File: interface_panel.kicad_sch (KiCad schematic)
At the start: 5 parts, among them J1 Conn_02x04_Odd_Even

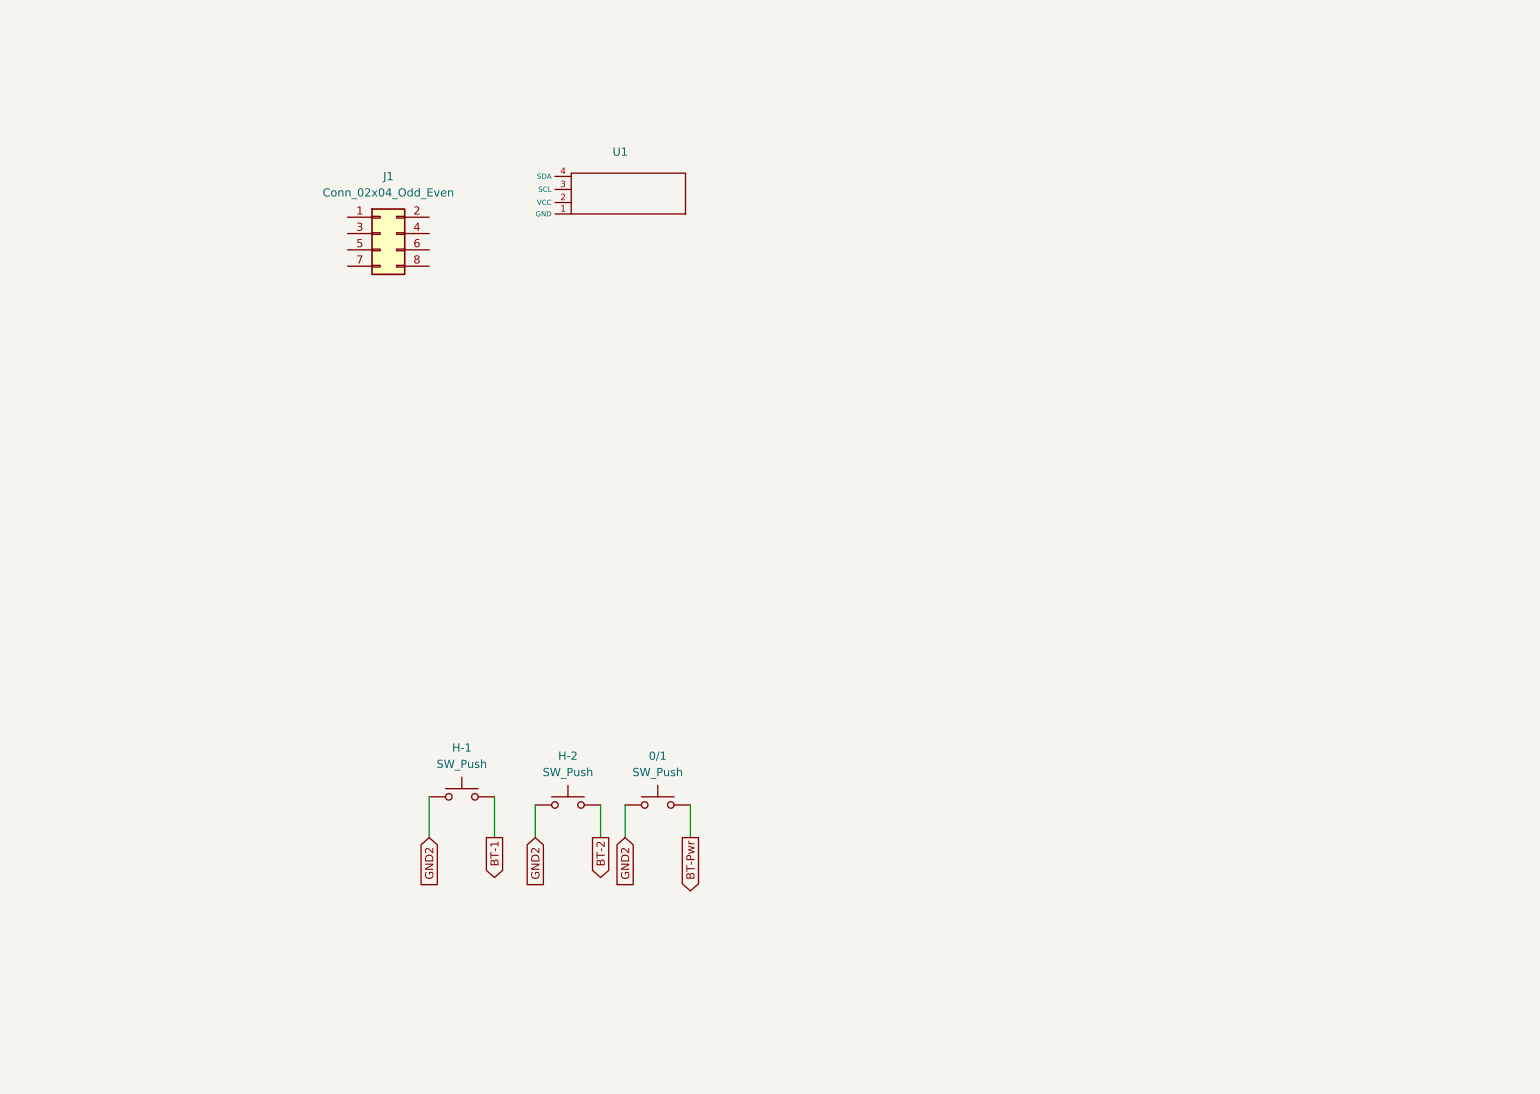
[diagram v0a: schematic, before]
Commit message: same
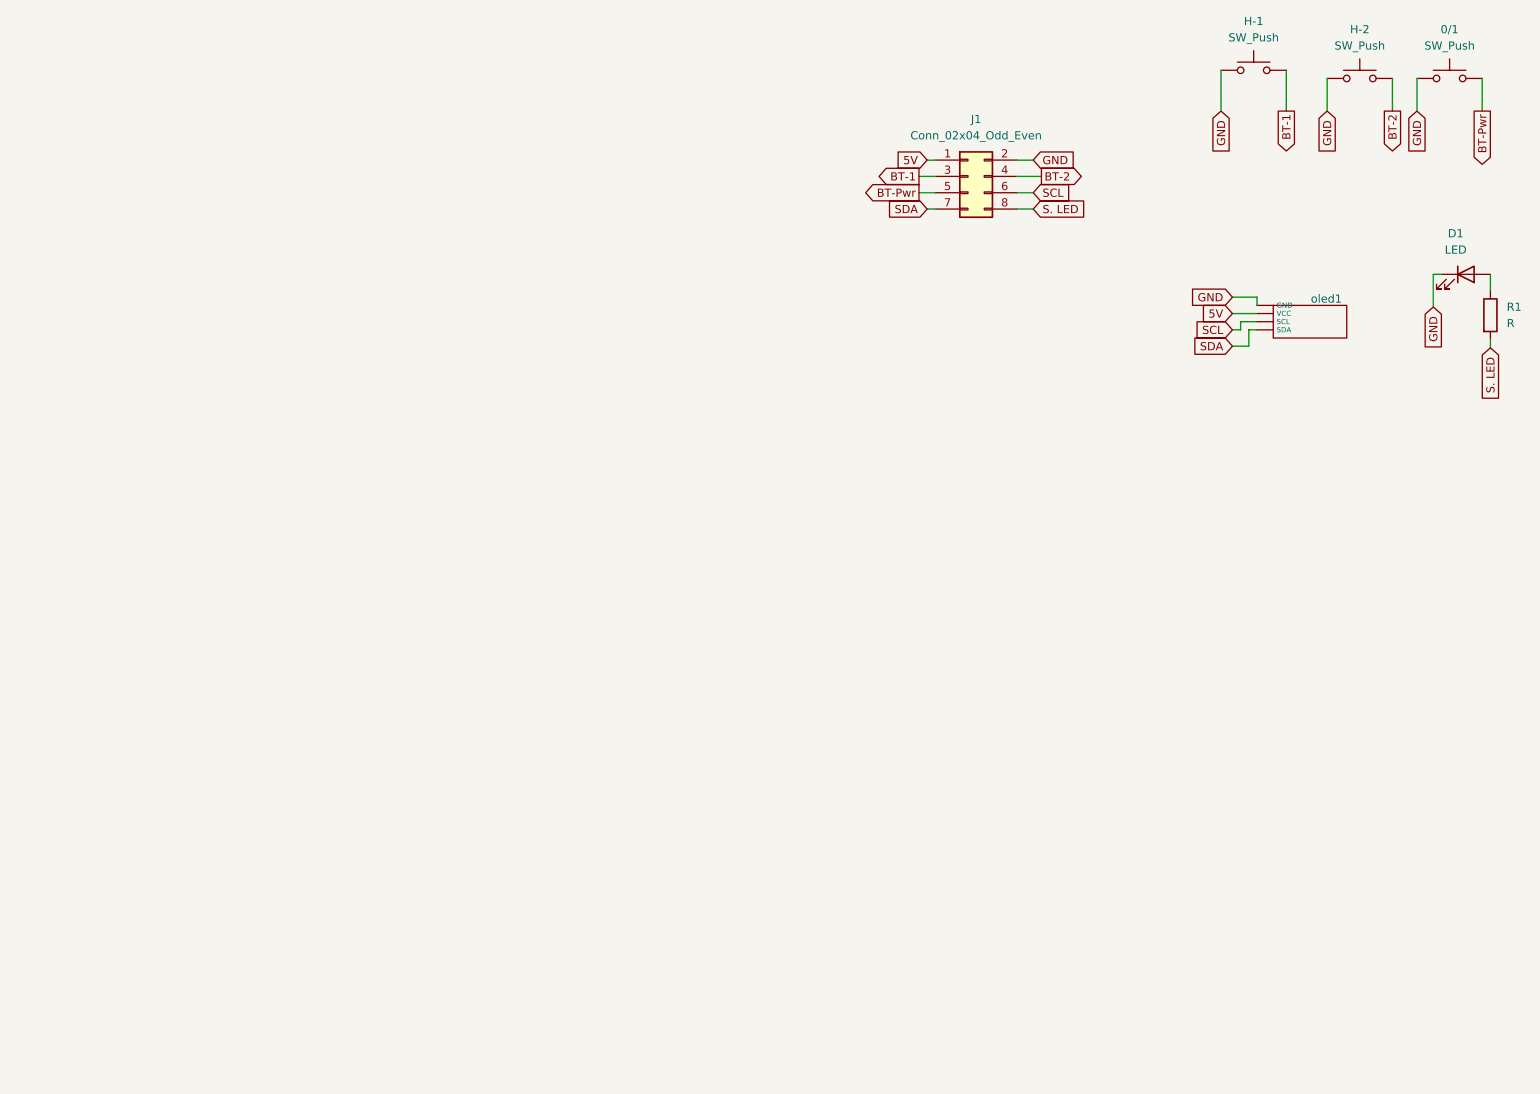
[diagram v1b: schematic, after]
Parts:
- added D1: LED, LED_THT:LED_D3.0mm, symbol Device:LED
- added R1: R, Resistor_THT:R_Axial_DIN0207_L6.3mm_D2.5mm_P7.62mm_Horizontal, symbol Device:R
- added oled1: ~, symbol New_Library:oled
- H-1, H-2: footprint (none) -> Button_Switch_THT:SW_PUSH_6mm
- J1: footprint (none) -> Connector_IDC:IDC-Header_2x04_P2.54mm_Vertical
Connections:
- net GND2 is gone; now on net GND: 0/1.1, H-1.1, H-2.1
- net BT-1: now also J1.3 (Pin_3)
- net BT-2: now also J1.4 (Pin_4)
- net BT-Pwr: now also J1.5 (Pin_5)
- net 5V: now reaches J1.1 (Pin_1)
- net 5V: now also oled1. (VCC)
- net GND: now reaches J1.2 (Pin_2)
- net GND: now also D1.1 (K), oled1. (VCC)
- net SCL: now reaches J1.6 (Pin_6)
- net SCL: now also oled1. (VCC)
- net SDA: now reaches J1.7 (Pin_7)
- net SDA: now also oled1. (VCC)
- net S. LED: now reaches J1.8 (Pin_8)
- net S. LED: now also R1.2
- new net: D1.2 (A), R1.1
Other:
- moved on the sheet: 0/1, H-1, H-2, J1

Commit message: PCB saved
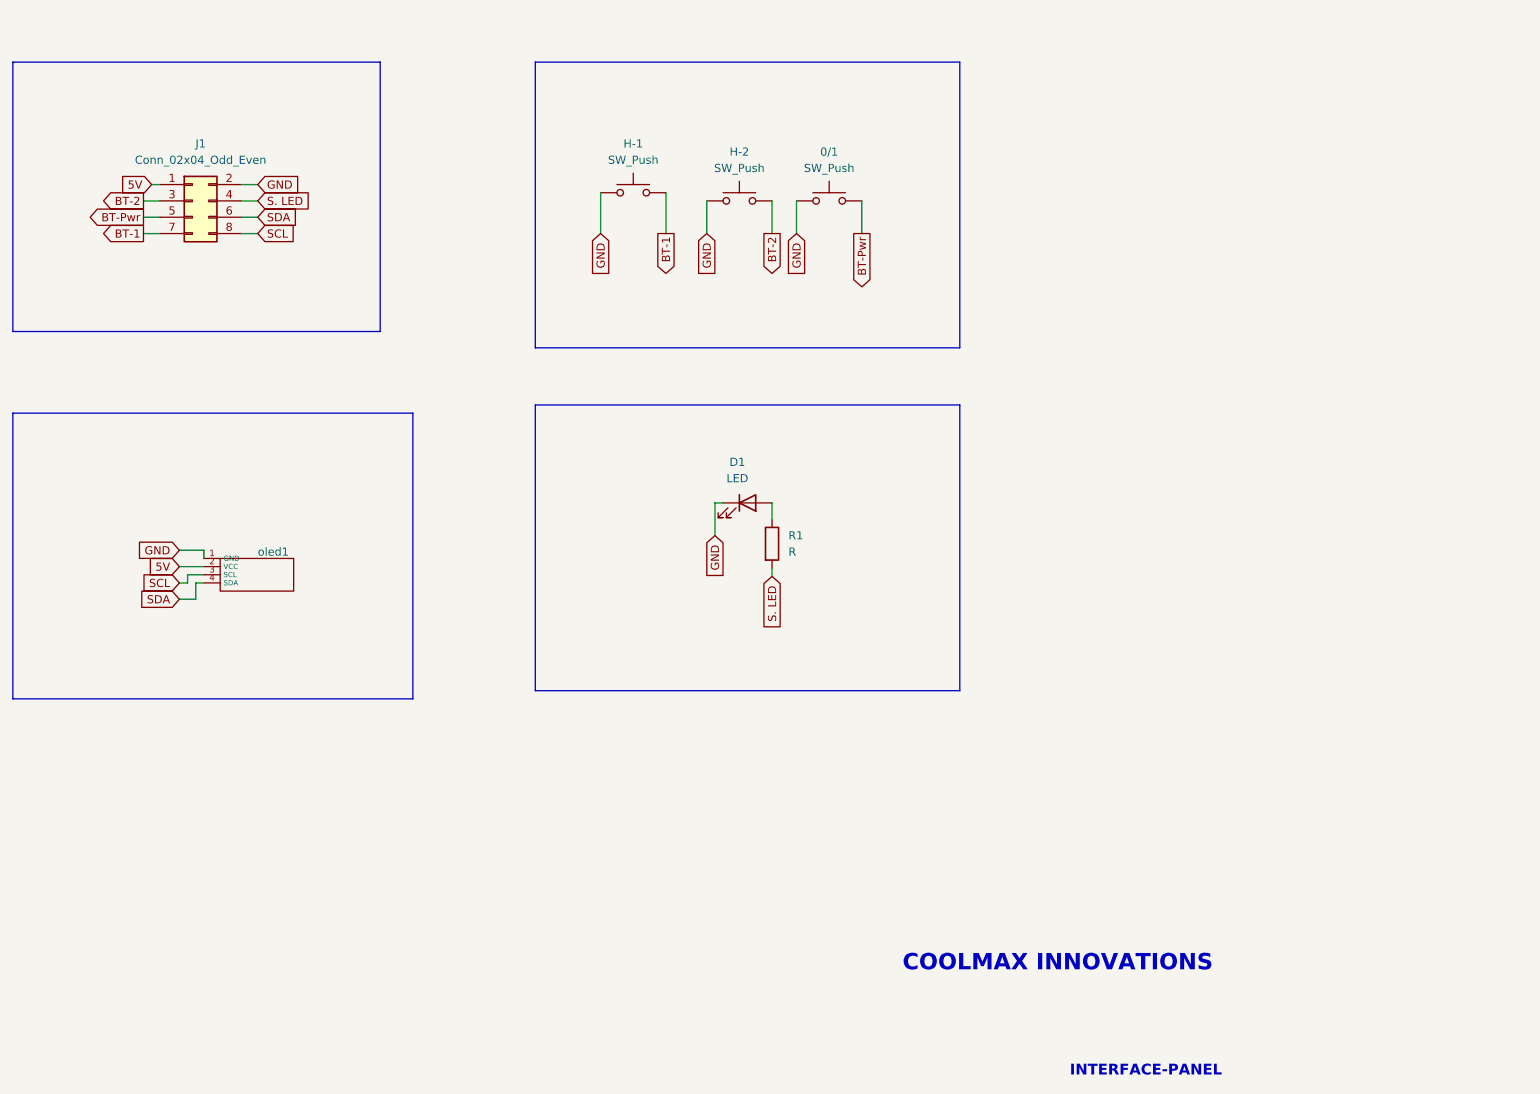
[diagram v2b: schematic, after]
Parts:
- 0/1: footprint (none) -> Button_Switch_THT:SW_PUSH_6mm
- oled1: footprint (none) -> oled0.9in:SSD1306-0.91-OLED-4pin-128x32
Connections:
- net 5V: now also oled1.2 (VCC); no longer oled1. (VCC)
- net BT-1: now also J1.7 (Pin_7); no longer J1.3 (Pin_3)
- net BT-2: now also J1.3 (Pin_3); no longer J1.4 (Pin_4)
- net GND: now also oled1.1 (GND); no longer oled1. (VCC)
- net S. LED: now also J1.4 (Pin_4); no longer J1.8 (Pin_8)
- net SCL: now also J1.8 (Pin_8), oled1.3 (SCL); no longer J1.6 (Pin_6), oled1. (VCC)
- net SDA: now also J1.6 (Pin_6), oled1.4 (SDA); no longer J1.7 (Pin_7), oled1. (VCC)
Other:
- note added: "COOLMAX INNOVATIONS"
- note added: "INTERFACE-PANEL"
- moved on the sheet: 0/1, D1, H-1, H-2, J1, R1

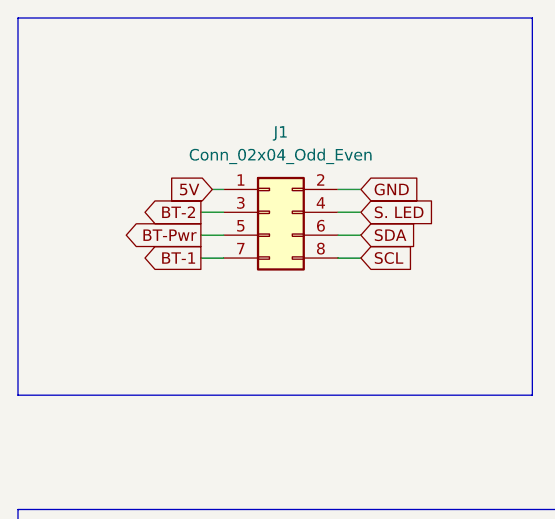
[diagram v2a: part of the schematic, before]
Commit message: panel_final
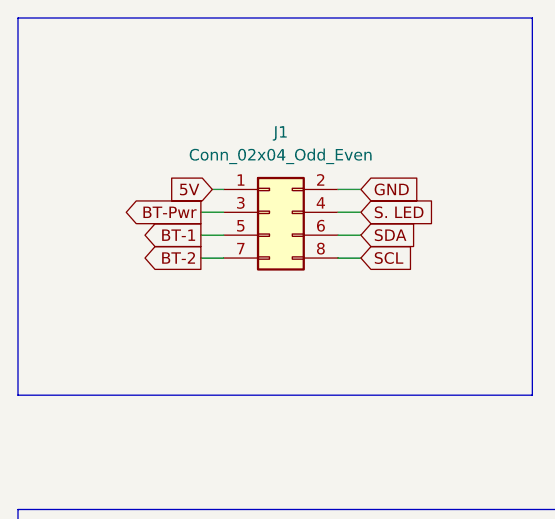
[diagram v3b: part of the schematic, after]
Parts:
- R1: footprint Resistor_THT:R_Axial_DIN0207_L6.3mm_D2.5mm_P7.62mm_Horizontal -> Resistor_THT:R_Axial_DIN0204_L3.6mm_D1.6mm_P5.08mm_Horizontal
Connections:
- net BT-1: now also J1.5 (Pin_5); no longer J1.7 (Pin_7)
- net BT-2: now also J1.7 (Pin_7); no longer J1.3 (Pin_3)
- net BT-Pwr: now also J1.3 (Pin_3); no longer J1.5 (Pin_5)
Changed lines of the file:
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@@
-		)
-	)
-	(global_label "GND"
-		(shape input)
-		(at 65.278 108.966 180)
-		(fields_autoplaced yes)
-		(effects
-			(font
-				(size 1.27 1.27)
-			)
-			(justify right)
-		)
-		(property "Intersheetrefs" "${INTERSHEET_REFS}"
-			(at 58.4223 108.966 0)
-			(effects
-				(font
-					(size 1.27 1.27)
-				)
-				(justify right)
-				(hide yes)
-			)
-		)
-	)
-	(global_label "S. LED"
-		(shape input)
-		(at 157.48 113.03 270)
-		(fields_autoplaced yes)
-		(effects
-			(font
-				(size 1.27 1.27)
-			)
-			(justify right)
-		)
-		(property "Intersheetrefs" "${INTERSHEET_REFS}"
-			(at 157.48 122.2442 90)
-			(effects
-				(font
-					(size 1.27 1.27)
-				)
-				(justify right)
-				(hide yes)
-			)
-		)
-	)
-	(global_label "GND"
-		(shape input)
-		(at 130.81 59.69 270)
-		(fields_autoplaced yes)
-		(effects
-			(font
-				(size 1.27 1.27)
-			)
-			(justify right)
-		)
-		(property "Intersheetrefs" "${INTERSHEET_REFS}"
-			(at 130.81 66.5457 90)
-			(effects
-				(font
-					(size 1.27 1.27)
-				)
-				(justify right)
-				(hide yes)
-			)
 		)
 	)
 	(global_label "BT-2"
 		(shape output)
-		(at 59.69 54.61 180)
-		(fields_autoplaced yes)
-		(effects
-			(font
-				(size 1.27 1.27)
-			)
-			(justify right)
-		)
-		(property "Intersheetrefs" "${INTERSHEET_REFS}"
-			(at 51.6853 54.61 0)
+		(at 59.69 59.69 180)
+		(fields_autoplaced yes)
+		(effects
+			(font
+				(size 1.27 1.27)
+			)
+			(justify right)
+		)
+		(property "Intersheetrefs" "${INTERSHEET_REFS}"
+			(at 51.6853 59.69 0)
 			(effects
 				(font
@@
 	(global_label "GND"
 		(shape input)
+		(at 65.278 108.966 180)
+		(fields_autoplaced yes)
+		(effects
+			(font
+				(size 1.27 1.27)
+			)
+			(justify right)
+		)
+		(property "Intersheetrefs" "${INTERSHEET_REFS}"
+			(at 58.4223 108.966 0)
+			(effects
+				(font
+					(size 1.27 1.27)
+				)
+				(justify right)
+				(hide yes)
+			)
+		)
+	)
+	(global_label "S. LED"
+		(shape input)
+		(at 157.48 113.03 270)
+		(fields_autoplaced yes)
+		(effects
+			(font
+				(size 1.27 1.27)
+			)
+			(justify right)
+		)
+		(property "Intersheetrefs" "${INTERSHEET_REFS}"
+			(at 157.48 122.2442 90)
+			(effects
+				(font
+					(size 1.27 1.27)
+				)
+				(justify right)
+				(hide yes)
+			)
+		)
+	)
+	(global_label "GND"
+		(shape input)
+		(at 130.81 59.69 270)
+		(fields_autoplaced yes)
+		(effects
+			(font
+				(size 1.27 1.27)
+			)
+			(justify right)
+		)
+		(property "Intersheetrefs" "${INTERSHEET_REFS}"
+			(at 130.81 66.5457 90)
+			(effects
+				(font
+					(size 1.27 1.27)
+				)
+				(justify right)
+				(hide yes)
+			)
+		)
+	)
+	(global_label "GND"
+		(shape input)
 		(at 161.29 59.69 270)
 		(fields_autoplaced yes)
@@
 				)
 				(justify left)
-				(hide yes)
-			)
-		)
-	)
-	(global_label "BT-Pwr"
-		(shape output)
-		(at 59.69 57.15 180)
-		(fields_autoplaced yes)
-		(effects
-			(font
-				(size 1.27 1.27)
-			)
-			(justify right)
-		)
-		(property "Intersheetrefs" "${INTERSHEET_REFS}"
-			(at 49.5081 57.15 0)
-			(effects
-				(font
-					(size 1.27 1.27)
-				)
-				(justify right)
 				(hide yes)
 			)
@@
 		)
 	)
-	(global_label "BT-1"
-		(shape output)
-		(at 59.69 59.69 180)
-		(fields_autoplaced yes)
-		(effects
-			(font
-				(size 1.27 1.27)
-			)
-			(justify right)
-		)
-		(property "Intersheetrefs" "${INTERSHEET_REFS}"
-			(at 51.6853 59.69 0)
-			(effects
-				(font
-					(size 1.27 1.27)
-				)
-				(justify right)
-				(hide yes)
-			)
-		)
-	)
 	(global_label "SCL"
 		(shape input)
@@
 		)
 	)
+	(global_label "BT-Pwr"
+		(shape output)
+		(at 59.69 54.61 180)
+		(fields_autoplaced yes)
+		(effects
+			(font
+				(size 1.27 1.27)
+			)
+			(justify right)
+		)
+		(property "Intersheetrefs" "${INTERSHEET_REFS}"
+			(at 49.5081 54.61 0)
+			(effects
+				(font
+					(size 1.27 1.27)
+				)
+				(justify right)
+				(hide yes)
+			)
+		)
+	)
 	(global_label "GND"
 		(shape input)
@@
 		(property "Intersheetrefs" "${INTERSHEET_REFS}"
 			(at 59.9947 111.506 0)
+			(effects
+				(font
+					(size 1.27 1.27)
+				)
+				(justify right)
+				(hide yes)
+			)
+		)
+	)
+	(global_label "BT-1"
+		(shape output)
+		(at 59.69 57.15 180)
+		(fields_autoplaced yes)
+		(effects
+			(font
+				(size 1.27 1.27)
+			)
+			(justify right)
+		)
+		(property "Intersheetrefs" "${INTERSHEET_REFS}"
+			(at 51.6853 57.15 0)
 			(effects
 				(font
@@
 			)
 		)
-		(property "Footprint" "Resistor_THT:R_Axial_DIN0207_L6.3mm_D2.5mm_P7.62mm_Horizontal"
+		(property "Footprint" "Resistor_THT:R_Axial_DIN0204_L3.6mm_D1.6mm_P5.08mm_Horizontal"
 			(at 155.702 107.95 90)
 			(effects
